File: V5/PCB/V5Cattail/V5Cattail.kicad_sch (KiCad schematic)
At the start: 8 parts, among them U11 ST-0277D00-052-142, U12 SRV05-4_C558418, U5 BMI270

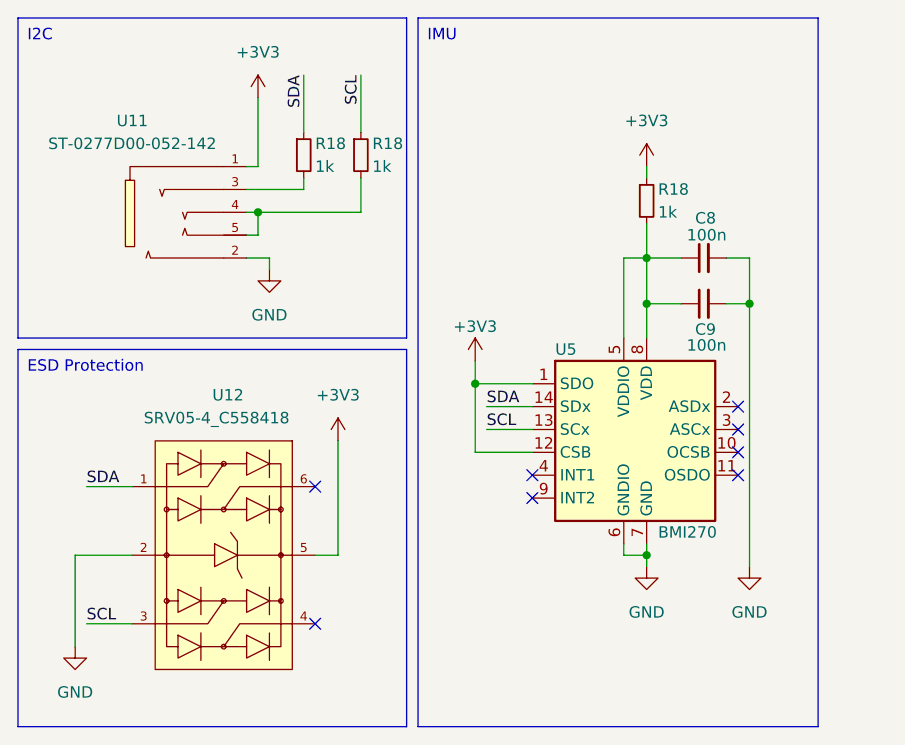
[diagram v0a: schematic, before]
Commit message: Overdue backup
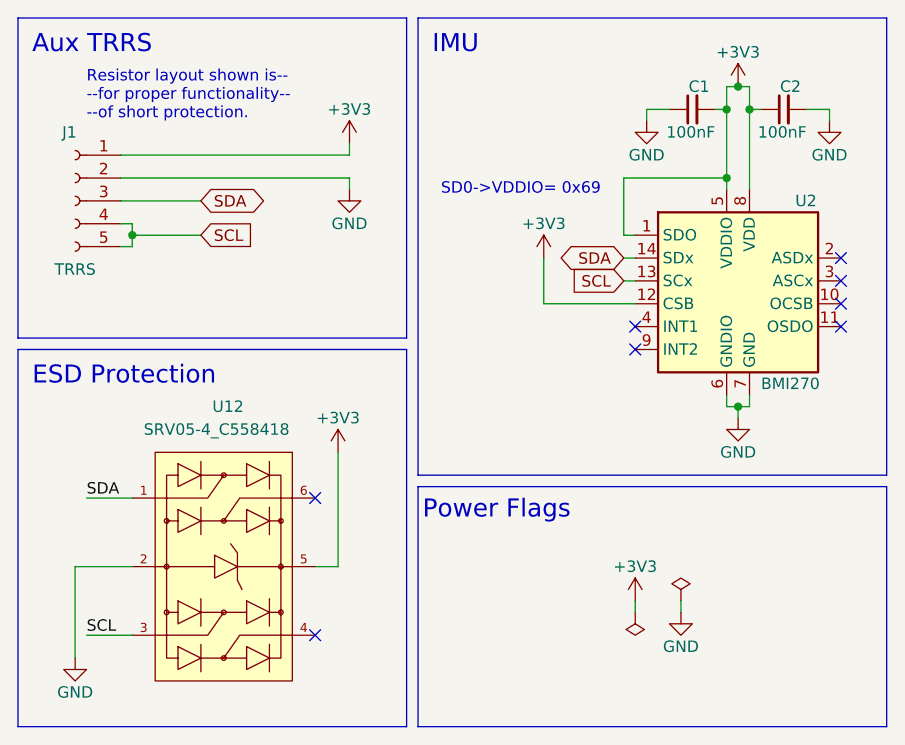
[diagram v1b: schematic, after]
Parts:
- removed C8, C9: 100n, Capacitor_SMD:C_0603_1608Metric, symbol CosmicLSM_Symbols:C_Small
- removed R18 (x3): 1k, Resistor_SMD:R_0603_1608Metric, symbol CosmicLSM_Symbols:R_Small
- removed U11: ST-0277D00-052-142, AUDIO-TH_ST-0277D00-052-142:AUDIO-TH_ST-0277D00-052-142, symbol ST-0277D00-052-142:ST-0277D00-052-142
- removed U5: BMI270, Package_LGA:Bosch_LGA-14_3x2.5mm_P0.5mm, symbol CosmicLSM_Symbols:BMI270
- added C1, C2: 100nF, LilypadVR:C_0603_1608Metric, symbol LilypadVR:C_Small
- added J1: TRRS, LilypadVR:AUDIO-TH_ST-0277D00-052-142, symbol LilypadVR:Conn_01x05_Socket
- added U2: BMI270, Package_LGA:Bosch_LGA-14_3x2.5mm_P0.5mm, symbol LilypadVR:BMI270
- U12: footprint SOT-23-6_L2.9-W1.6-P0.95-LS2.8-BL:SOT-23-6_L2.9-W1.6-P0.95-LS2.8-BL -> footprint:SOT-23-6_L2.9-W1.6-P0.95-LS2.8-BL; symbol SRV05-4_C558418:SRV05-4_C558418 -> LilypadVR:SRV05-4_C558418
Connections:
- net +3V3: now also C1.2, C2.1, J1.1 (Pin_1), U2.1 (SDO), U2.12 (CSB), U2.5 (VDDIO), U2.8 (VDD)
- net GND: now also C1.1, C2.2, J1.2 (Pin_2), U2.6 (GNDIO), U2.7 (GND)
- net SCL: now also J1.4 (Pin_4), J1.5 (Pin_5), U2.13 (SCx)
- net SDA: now also J1.3 (Pin_3), U2.14 (SDx)
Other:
- note added: "Power Flags"
- note added: "Resistor layout shown is-- --for proper functionality-- --of short protection."
- note added: "SD0->VDDIO= 0x69"
- moved on the sheet: U12
